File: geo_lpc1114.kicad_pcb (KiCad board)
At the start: 2 copper layers, 129.4 x 75.1 mm, 147 parts, among them J1 CN_SWD, J10 Screw_Terminal_01x02, J11 Screw_Terminal_01x02, J12 Screw_Terminal_01x02, J13 Screw_Terminal_01x02, J14 Screw_Terminal_01x02, J15 Screw_Terminal_01x02, J16 Screw_Terminal_01x02, J17 Screw_Terminal_01x02, J18 USB_B, J19 MJ-179PH, J2 Screw_Terminal_01x02, J3 Screw_Terminal_01x02, J4 Screw_Terminal_01x02, J5 Screw_Terminal_01x02, J6 Screw_Terminal_01x02, J7 Screw_Terminal_01x02, J8 Screw_Terminal_01x02, J9 Screw_Terminal_01x02, M3 MountingHole_3.2mm_M3, Q1 S8550, Q2 S8550, Q3 S8550, Q4 S8550, Q5 S8550, Q6 S8550, Q7 S8550, Q8 S8550, SW1 SW, U1 LPC1114FN28-102, U10 LPC1114FDH28-102, U11 CH340N, U12 LM2940T-3.3, U2 HX711, U3 HX711, U4 HX711, U5 HX711, U6 HX711, U7 HX711, U8 HX711, U9 HX711, Y1 ZZT 12.0MT-22P

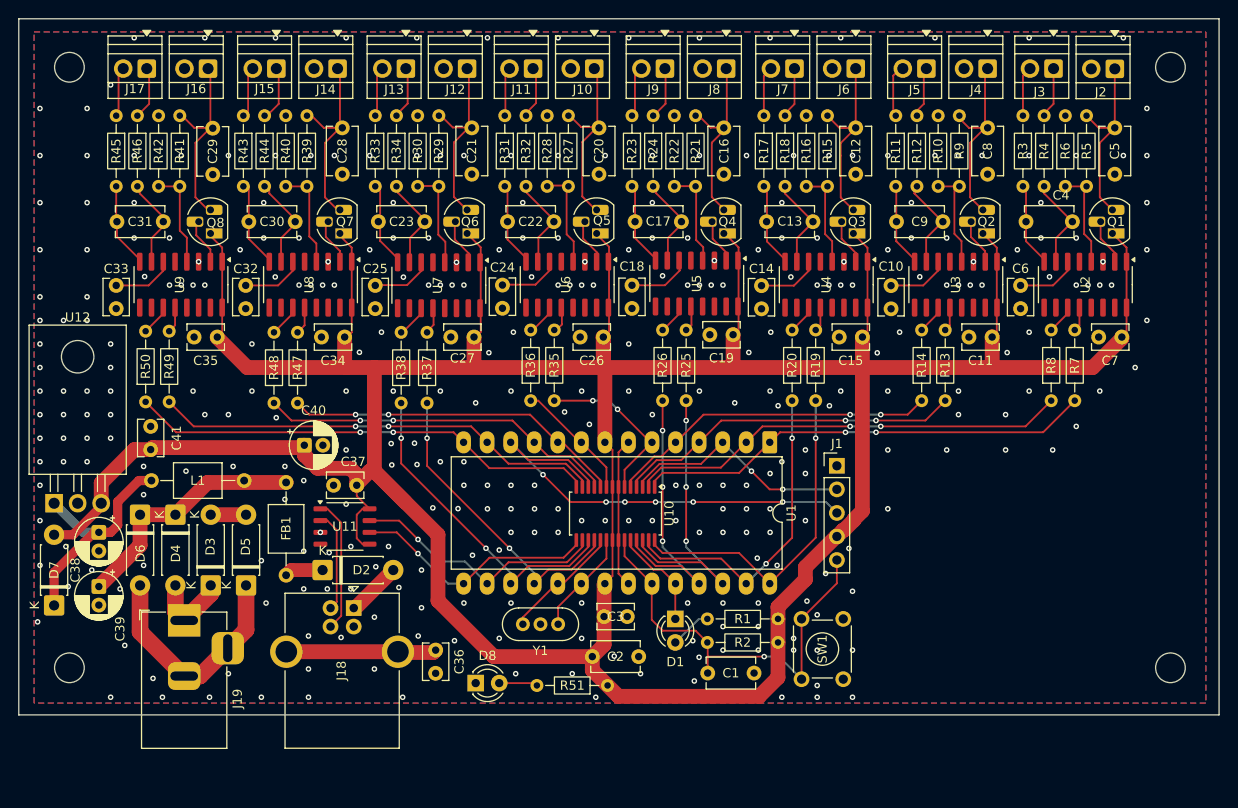
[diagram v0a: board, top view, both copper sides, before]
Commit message: fubriaction version 2024/09 1st week
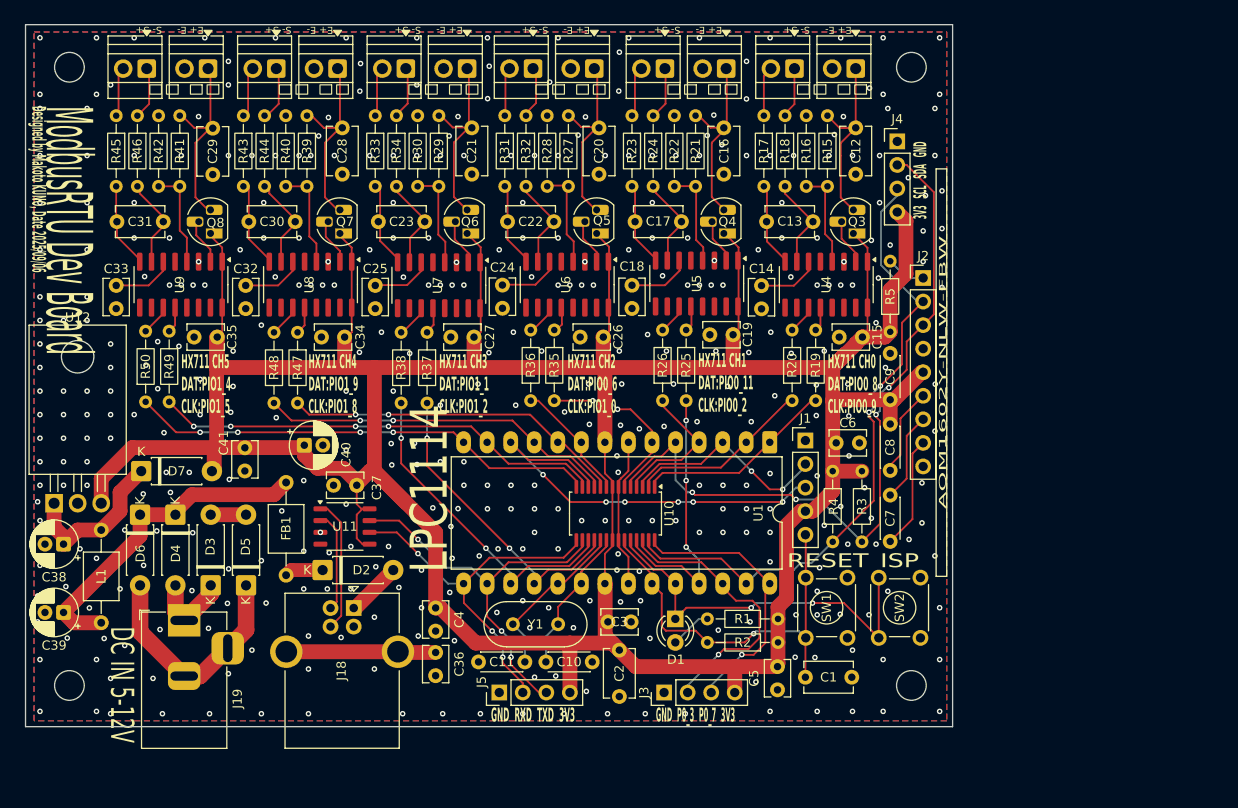
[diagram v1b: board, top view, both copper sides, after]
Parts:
- removed D8: LED, LED_THT:LED_D3.0mm
- removed Q1, Q2: S8550, Package_TO_SOT_THT:TO-92_HandSolder
- removed R10, R6, R9: 20k, Resistor_THT:R_Axial_DIN0204_L3.6mm_D1.6mm_P7.62mm_Horizontal
- removed R11, R12: 100, Resistor_THT:R_Axial_DIN0204_L3.6mm_D1.6mm_P7.62mm_Horizontal
- removed R13, R14, R7, R8: 20, Resistor_THT:R_Axial_DIN0204_L3.6mm_D1.6mm_P7.62mm_Horizontal
- removed R51: 10k, Resistor_THT:R_Axial_DIN0204_L3.6mm_D1.6mm_P7.62mm_Horizontal
- removed U2, U3: HX711, Package_SO:SOIC-16_3.9x9.9mm_P1.27mm
- added SW2: SW, Button_Switch_THT:SW_TH_Tactile_Omron_B3F-100x, F.Cu at (176.2, 121.7)
- C10, C11: value 0.1μF 50V X7R -> 22pF; footprint Capacitor_THT:C_Disc_D3.8mm_W2.6mm_P2.50mm -> Capacitor_THT:C_Disc_D4.3mm_W1.9mm_P5.00mm
- C4, C5: value 10μF 16V X7R -> 0.1μF 50V X7R; footprint Capacitor_THT:C_Disc_D5.1mm_W3.2mm_P5.00mm -> Capacitor_THT:C_Disc_D3.8mm_W2.6mm_P2.50mm
- C7: value 0.1μF 50V X7R -> 1μF 50V X7R; footprint Capacitor_THT:C_Disc_D3.8mm_W2.6mm_P2.50mm -> Capacitor_THT:C_Disc_D4.3mm_W1.9mm_P5.00mm
- C8, C9: value 10μF 16V X7R -> 1μF 50V X7R; footprint Capacitor_THT:C_Disc_D5.1mm_W3.2mm_P5.00mm -> Capacitor_THT:C_Disc_D4.3mm_W1.9mm_P5.00mm
- J2: value Screw_Terminal_01x02 -> AQM1602Y-NLW-FBW; footprint TerminalBlock:TerminalBlock_Xinya_XY308-2.54-2P_1x02_P2.54mm_Horizontal -> Connector_PinHeader_2.54mm:PinHeader_1x09_P2.54mm_Vertical
- J3: value Screw_Terminal_01x02 -> GPIO_Header; footprint TerminalBlock:TerminalBlock_Xinya_XY308-2.54-2P_1x02_P2.54mm_Horizontal -> Connector_PinHeader_2.54mm:PinHeader_1x04_P2.54mm_Vertical
- J4: value Screw_Terminal_01x02 -> I2C_Header; footprint TerminalBlock:TerminalBlock_Xinya_XY308-2.54-2P_1x02_P2.54mm_Horizontal -> Connector_PinHeader_2.54mm:PinHeader_1x04_P2.54mm_Vertical
- J5: value Screw_Terminal_01x02 -> UART_Header; footprint TerminalBlock:TerminalBlock_Xinya_XY308-2.54-2P_1x02_P2.54mm_Horizontal -> Connector_PinHeader_2.54mm:PinHeader_1x04_P2.54mm_Vertical
- R1: value 4.7k -> 10k
- R3, R4: value 100 -> 10k
- R5: value 20k -> 10k
- Y1: value ZZT 12.0MT-22P -> 12MHz; footprint Crystal:Crystal_HC52-U-3Pin_Vertical -> Crystal:Crystal_HC49-U_Vertical
- moved J5 81.5 mm to (130.8, 134.1), turned to 90 degrees
- moved J3 79.3 mm to (148.6, 134.1), turned to 90 degrees
- moved C4 76.1 mm to (124.0, 125.0), turned to -90 degrees
- moved C5 68.6 mm to (160.8, 131.3)
- moved C11 59.3 mm to (133.6, 130.8), turned to 180 degrees
- moved C10 55.1 mm to (135.8, 130.8), turned to 0 degrees
- moved R4 44.6 mm to (166.8, 110.2)
- moved R3 42.1 mm to (169.9, 110.2)
- moved C8 38.4 mm to (173.0, 110.2), turned to 90 degrees
- moved C7 31.5 mm to (173.0, 117.8), turned to 90 degrees
- moved J2 30.6 mm to (176.5, 89.4), turned to 0 degrees
- moved REF** 28.0 mm to (175.3, 133.3)
- moved REF** 27.9 mm to (175.3, 66.7)
- moved R5 26.4 mm to (173.0, 95.2)
- moved C6 26.1 mm to (167.2, 107.2), turned to 0 degrees
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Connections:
- net LED renamed ISP/LED
- C10 pad 1: Net-(U3-VBG) -> XTAL_IN
- C11 pad 1: GND -> XTAL_OUT
- C11 pad 2: +3V3 -> GND
- C4 pad 1: Net-(U2-INA+) -> +3V3
- C4 pad 2: Net-(U2-INA-) -> GND
- C5 pad 1: Net-(J2-Pin_1) -> +3V3
- C6 pad 1: Net-(U2-VBG) -> +3V3
- C7 pad 1: GND -> Net-(J2-Pin_8)
- C7 pad 2: +3V3 -> Net-(J2-Pin_7)
- C8 pad 1: Net-(J4-Pin_1) -> Net-(J2-Pin_6)
- C8 pad 2: GND -> +3V3
- C9 pad 1: Net-(U3-INA+) -> +3V3
- C9 pad 2: Net-(U3-INA-) -> GND
- J2 pad 2: GND -> I2C_SCL
- J3 pad 1: Net-(J3-Pin_1) -> GND
- J3 pad 2: Net-(J3-Pin_2) -> PIO0_3
- J4 pad 1: Net-(J4-Pin_1) -> GND
- J4 pad 2: GND -> I2C_SDA
- J5 pad 1: Net-(J5-Pin_1) -> GND
- J5 pad 2: Net-(J5-Pin_2) -> UART_RX
- R19 pad 2: HX711_DAT_2 -> HX711_DAT_0
- R20 pad 1: HX711_CLK_2 -> HX711_CLK_0
- R25 pad 2: HX711_DAT_3 -> HX711_DAT_1
- R26 pad 1: HX711_CLK_3 -> HX711_CLK_1
- R3 pad 1: Net-(J3-Pin_2) -> +3V3
- R3 pad 2: Net-(U2-INA+) -> I2C_SDA
- R35 pad 2: HX711_DAT_4 -> HX711_DAT_2
- R36 pad 1: HX711_CLK_4 -> HX711_CLK_2
- R37 pad 2: HX711_DAT_6 -> HX711_DAT_4
- R38 pad 1: HX711_CLK_6 -> HX711_CLK_4
- R4 pad 1: Net-(J3-Pin_1) -> +3V3
- R4 pad 2: Net-(U2-INA-) -> I2C_SCL
- R47 pad 2: HX711_DAT_5 -> HX711_DAT_3
- R48 pad 1: HX711_CLK_5 -> HX711_CLK_3
- R49 pad 2: HX711_DAT_7 -> HX711_DAT_5
- R5 pad 1: Net-(U2-VFB) -> +3V3
- R50 pad 1: HX711_CLK_7 -> HX711_CLK_5
- U1 pad 10: HX711_DAT_5 -> HX711_DAT_3
- U1 pad 11: HX711_CLK_5 -> HX711_CLK_3
- U1 pad 13: HX711_DAT_7 -> HX711_DAT_5
- U1 pad 14: HX711_CLK_7 -> HX711_CLK_5
- U1 pad 17: HX711_CLK_6 -> HX711_CLK_4
- U1 pad 18: HX711_DAT_6 -> HX711_DAT_4
- U1 pad 25: HX711_CLK_3 -> HX711_DAT_1
- U1 pad 26: HX711_DAT_3 -> PIO0_3
- U1 pad 27: HX711_CLK_2 -> I2C_SCL
- U1 pad 28: HX711_DAT_2 -> PIO0_7
- U1 pad 4: HX711_DAT_1 -> HX711_CLK_1
- U1 pad 5: HX711_CLK_1 -> I2C_SDA
- U1 pad 6: HX711_DAT_4 -> HX711_DAT_2
- U1 pad 9: HX711_CLK_4 -> HX711_CLK_2
- U10 pad 10: HX711_DAT_5 -> HX711_DAT_3
- U10 pad 11: HX711_CLK_5 -> HX711_CLK_3
- U10 pad 13: HX711_DAT_7 -> HX711_DAT_5
- U10 pad 14: HX711_CLK_7 -> HX711_CLK_5
- U10 pad 17: HX711_CLK_6 -> HX711_CLK_4
- U10 pad 18: HX711_DAT_6 -> HX711_DAT_4
- U10 pad 25: HX711_CLK_3 -> HX711_DAT_1
- U10 pad 26: HX711_DAT_3 -> PIO0_3
- U10 pad 27: HX711_CLK_2 -> I2C_SCL
- U10 pad 28: HX711_DAT_2 -> PIO0_7
- U10 pad 4: HX711_DAT_1 -> HX711_CLK_1
- U10 pad 5: HX711_CLK_1 -> I2C_SDA
- U10 pad 6: HX711_DAT_4 -> HX711_DAT_2
- U10 pad 9: HX711_CLK_4 -> HX711_CLK_2
- Y1 pad 1: XTAL_IN -> XTAL_OUT
- Y1 pad 2: GND -> XTAL_IN
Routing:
- net I2C_SDA: track 0.00 -> 80.8 mm, vias 0 -> 4
- net I2C_SCL: track 0.00 -> 69.6 mm, vias 0 -> 2
- net HX711_CLK_7: track 50.7 -> 0.00 mm, vias 2 -> 0
- net HX711_DAT_7: track 48.8 -> 0.00 mm, vias 2 -> 0
- net HX711_CLK_6: track 35.1 -> 0.00 mm, vias 2 -> 0
- net HX711_DAT_6: track 33.1 -> 0.00 mm, vias 2 -> 0
- net ISP/LED: track 11.0 -> 41.8 mm, vias 0 -> 2
- net PIO0_3: track 0.00 -> 30.2 mm, vias 0 -> 1
- net PIO0_7: track 0.00 -> 29.8 mm, vias 0 -> 1
- net HX711_CLK_0: track 47.7 -> 19.8 mm, vias 2 -> 0
- net HX711_DAT_0: track 49.5 -> 21.6 mm, vias 2 -> 0
- net HX711_CLK_4: track 14.0 -> 35.1 mm, vias 0 -> 2
- net HX711_CLK_2: track 34.7 -> 14.0 mm, vias 2 -> 0
- net HX711_CLK_1: track 35.7 -> 15.3 mm, vias 2 -> 0
- net Net-(J4-Pin_1): track 20.0 -> 0.00 mm
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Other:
- board size 129.4 x 75.1 mm -> 100 x 75.7 mm
- board text added: "3V3 SCL SDA GND"
- board text added: "AQM1602Y-NLW-FBW"
- board text added: "DC IN 5-12V"
- board text added: "Designed by Makoto KUNO, Date 2025/09/06"
- board text added: "E+ E- S- S+"
- board text added: "GND P0_3 P0_7 3V3"
- board text added: "GND RXD TXD 3V3"
- board text added: "HX711 CH0 DAT:PIO0_8 CLK:PIO0_9"
- board text added: "HX711 CH1 DAT:PIO0_11 CLK:PIO0_2"
- board text added: "HX711 CH2 DAT:PIO0_6 CLK:PIO1_0"
- board text added: "HX711 CH3 DAT:PIO1_1 CLK:PIO1_2"
- board text added: "HX711 CH4 DAT:PIO1_9 CLK:PIO1_8"
- board text added: "HX711 CH5 DAT:PIO1_4 CLK:PIO1_5"
- board text added: "ISP"
- board text added: "LPC1114"
- board text added: "ModbusRTU Dev Board"
- board text added: "RESET"
- board text added: "赤黒 白緑"
